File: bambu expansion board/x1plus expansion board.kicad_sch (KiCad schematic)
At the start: 25 parts, among them CN1 USB-CON-AF-MH4, CN2 USB-CON-AF-MH4, CN3 USB-CON-AF-MH4, U1 LAN9514-JZX-TR, U2 TPS54202DDCR, U3 AMS1117-3.3, U4 HC913550A-M899-A, U5 FT2232HL

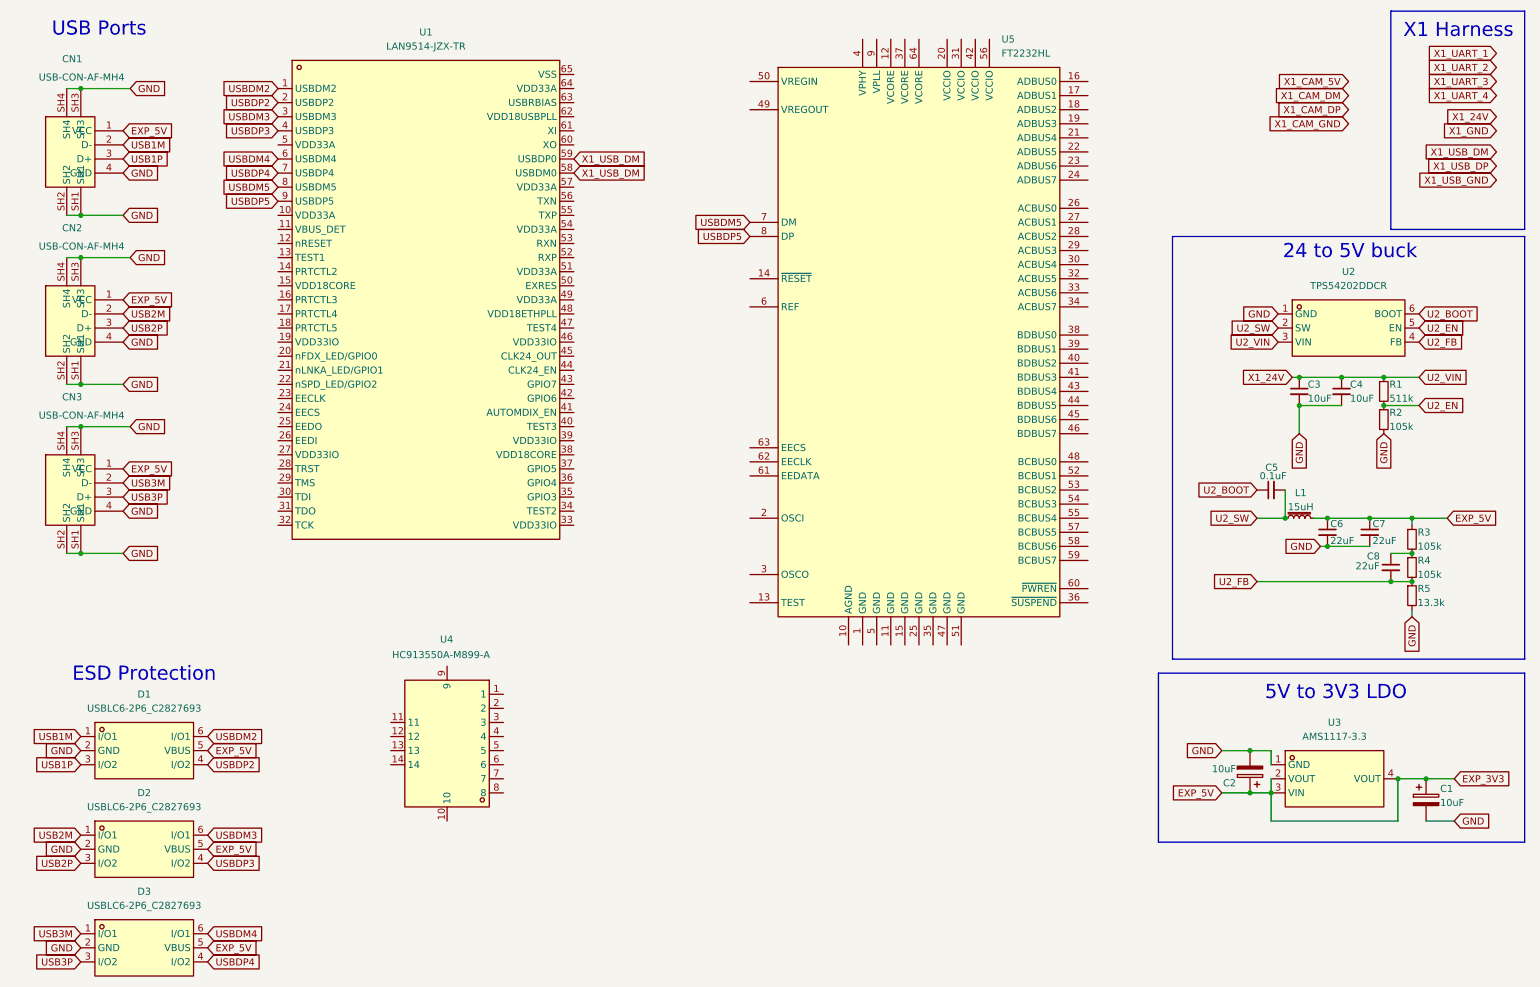
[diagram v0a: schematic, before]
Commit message: datasheets
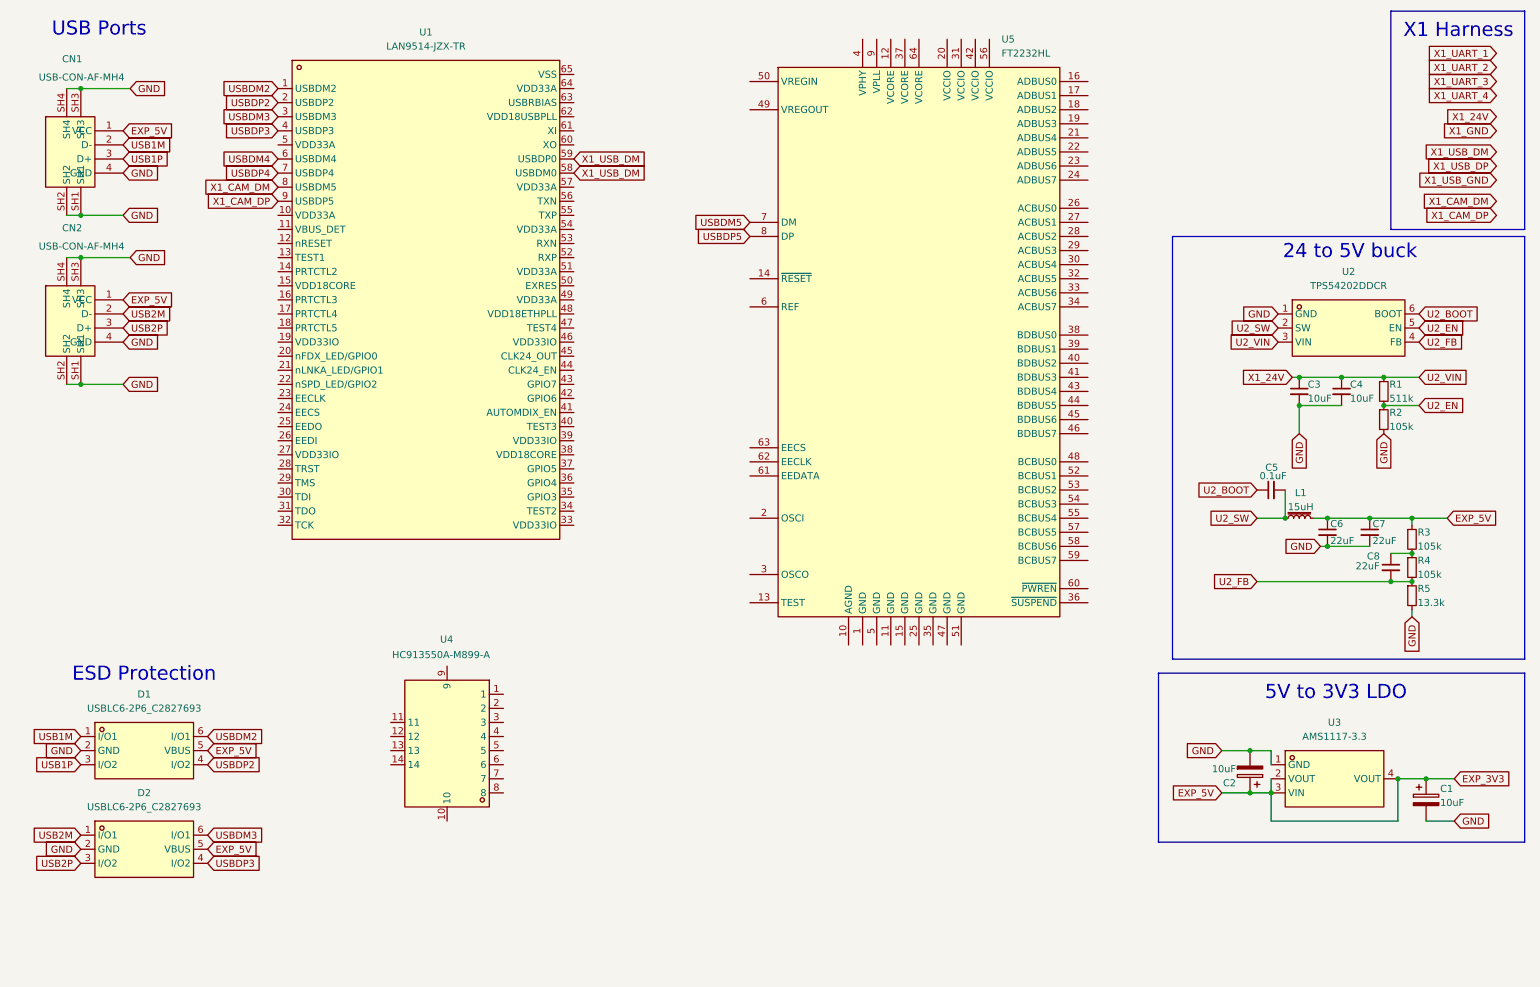
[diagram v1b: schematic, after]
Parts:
- removed CN3: USB-CON-AF-MH4, easyeda2kicad:USB-A-SMD_AF-MH4, symbol easyeda2kicad:USB-CON-AF-MH4
- removed D3: USBLC6-2P6_C2827693, easyeda2kicad:SOT-666-6_L1.6-W1.2-P0.50-LS1.6-BL, symbol easyeda2kicad:USBLC6-2P6_C2827693
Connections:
- net USBDM5: no longer U1.8 (USBDM5)
- net USBDP5: no longer U1.9 (USBDP5)
- net X1_CAM_DM: now also U1.8 (USBDM5)
- net X1_CAM_DP: now also U1.9 (USBDP5)
